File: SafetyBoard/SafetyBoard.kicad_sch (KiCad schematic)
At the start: 0 parts

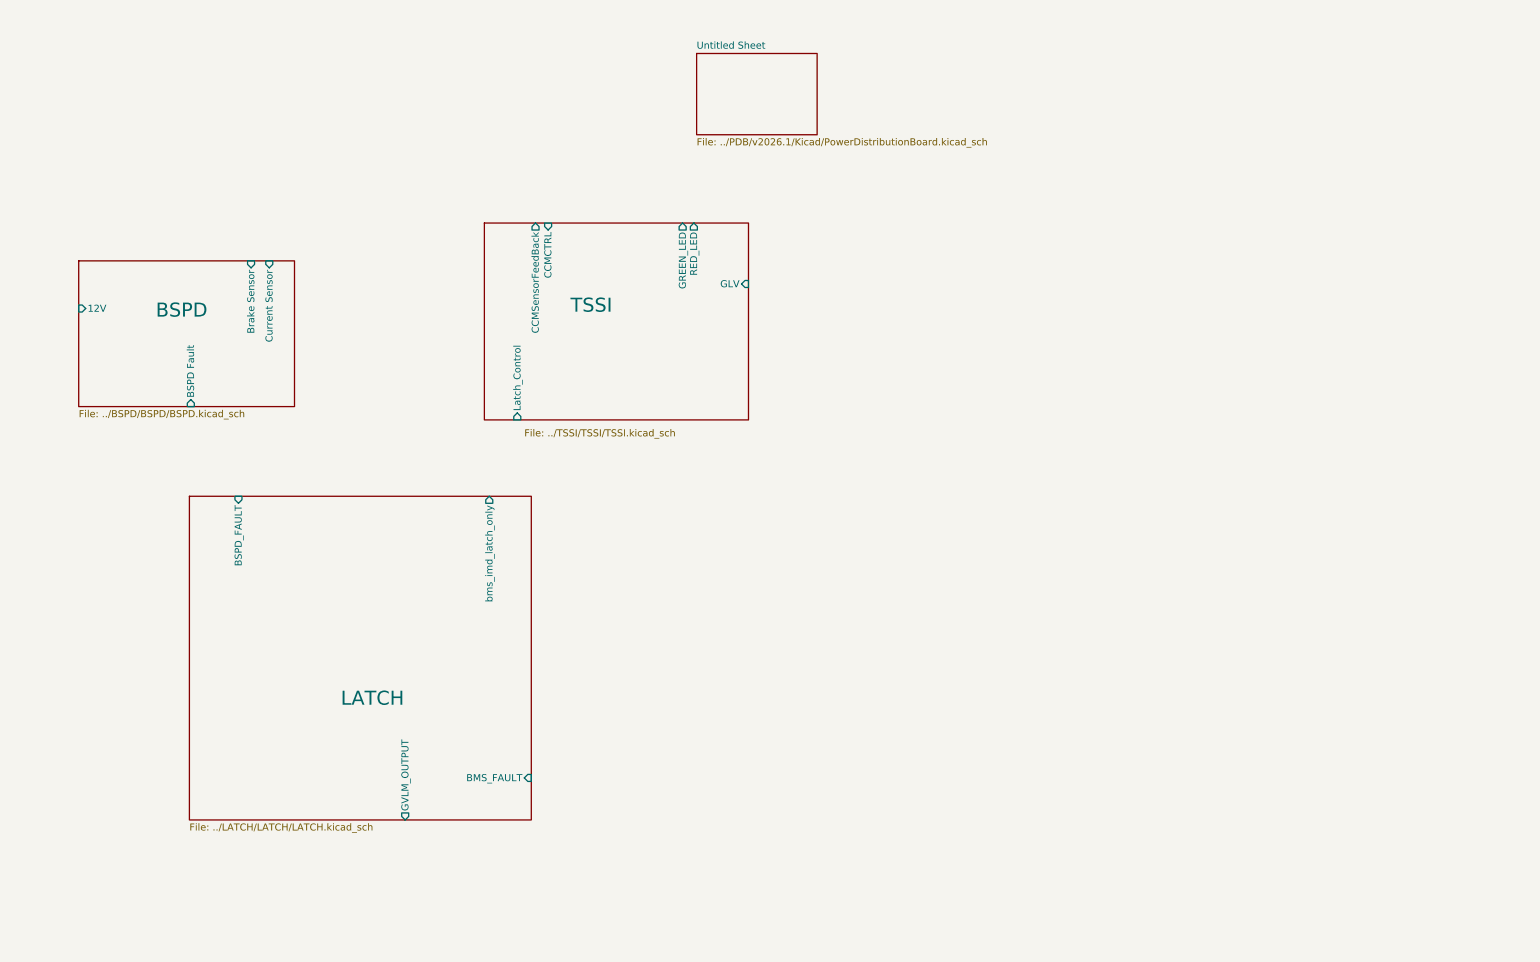
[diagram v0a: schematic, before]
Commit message: day 2 grind
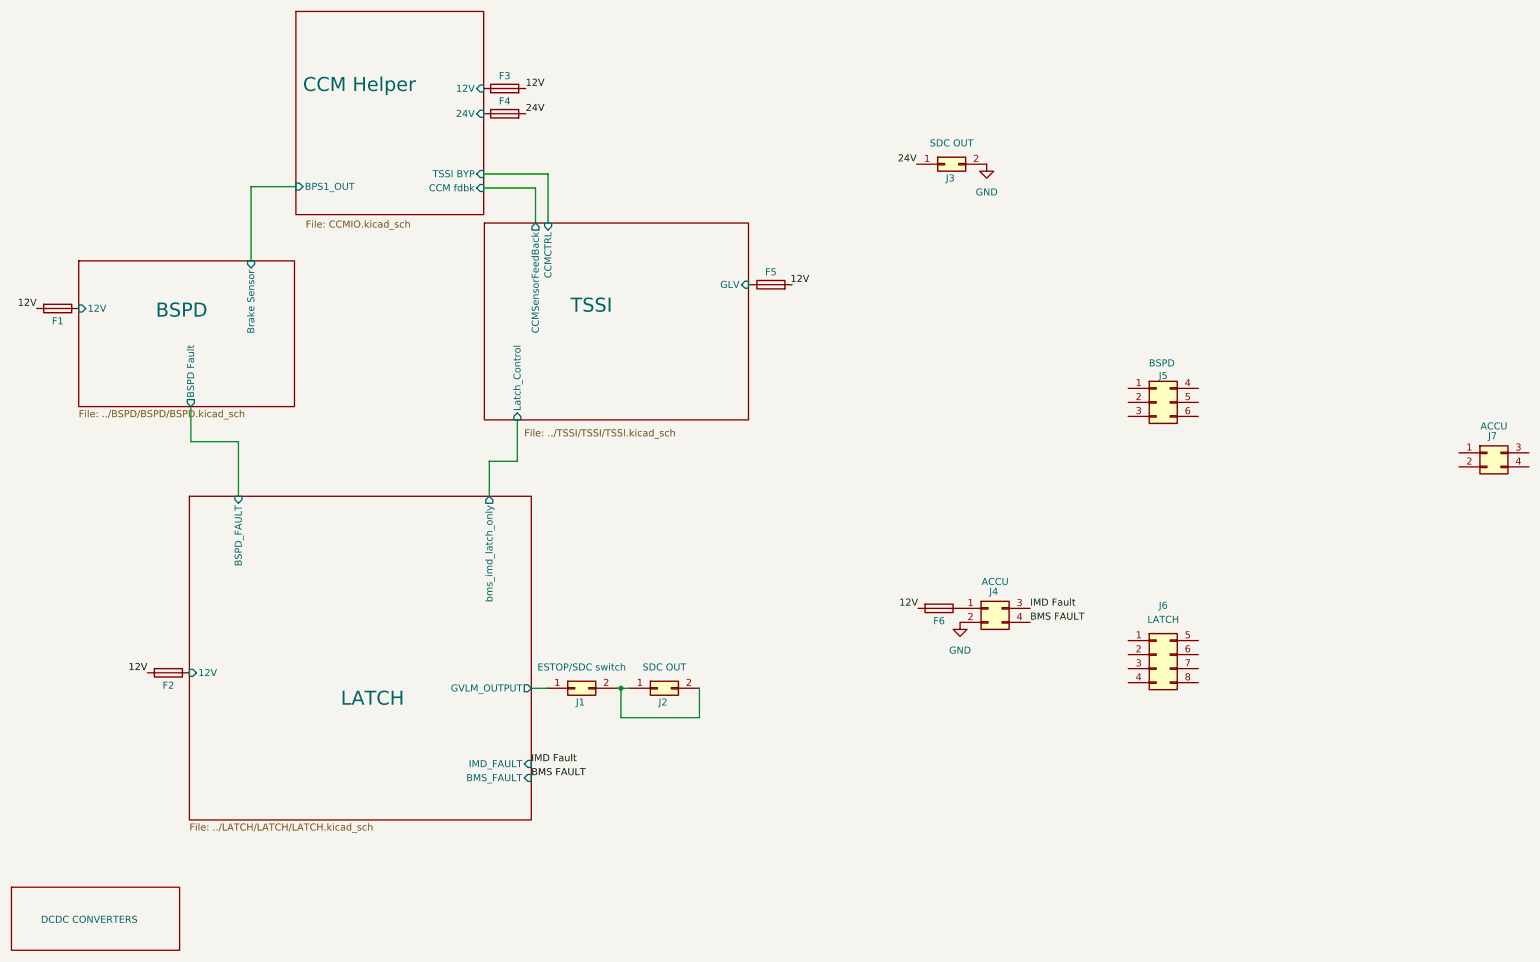
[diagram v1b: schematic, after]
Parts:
- added F1, F2, F3, F4, F5, F6: ~, 0footprints:FUSE_3522-2, symbol Device:Fuse
- added J1: ESTOP/SDC switch, 0footprints:Molex_Mini-Fit_Jr_5566-02A_2x01_P4.20mm_Vertical, symbol Connector_Generic:Conn_02x01
- added J2, J3: SDC OUT, 0footprints:Molex_Mini-Fit_Jr_5566-02A_2x01_P4.20mm_Vertical, symbol Connector_Generic:Conn_02x01
- added J4, J7: ACCU, 0footprints:Molex_Mini-Fit_Jr_5566-04A_2x02_P4.20mm_Vertical, symbol Connector_Generic:Conn_02x02_Top_Bottom
- added J5: BSPD, 0footprints:Molex_Mini-Fit_Jr_5566-06A_2x03_P4.20mm_Vertical, symbol Connector_Generic:Conn_02x03_Top_Bottom
- added J6: LATCH, 0footprints:Molex_Mini-Fit_Jr_5566-08A_2x04_P4.20mm_Vertical, symbol Connector_Generic:Conn_02x04_Top_Bottom
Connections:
- net BSPD/12V: now also F1.1
- net LATCH/GVLM_OUTPUT: now also J1.1 (Pin_1)
- net TSSI/GLV: now also F5.1
- new net: F6.1, J4.1 (Pin_1)
- new net: J1.2 (Pin_2), J2.1 (Pin_1), J2.2 (Pin_2)
- new net 12V: F1.2, F2.2, F3.2, F5.2, F6.2
- new net 24V: F4.2, J3.1 (Pin_1)
- new net BMS FAULT: J4.4 (Pin_4)
- new net CCM Helper/12V: F3.1
- new net CCM Helper/24V: F4.1
- new net GND: J3.2 (Pin_2), J4.2 (Pin_2)
- new net IMD Fault: J4.3 (Pin_3)
- new net LATCH/12V: F2.1
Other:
- removed sheet Untitled Sheet
- added sheet CCM Helper (CCMIO.kicad_sch)
- added sheet DCDC CONVERTERS (./24V DC-DC Converter 2/24V DC-DC Converter.kicad_sch)
- sheet BSPD ports: added none; removed Current Sensor
- sheet LATCH ports: added 12V, IMD_FAULT; removed none
- sheet TSSI ports: added none; removed GREEN_LED, RED_LED
